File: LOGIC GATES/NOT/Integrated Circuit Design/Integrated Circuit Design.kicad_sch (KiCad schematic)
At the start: 13 parts, among them J1 Conn_01x03_Socket, J2 Conn_01x03_Socket, J3 Conn_01x03_Socket, Q1 QM6006D, Q2 QM6006D, Q3 QM6006D, U1 4011

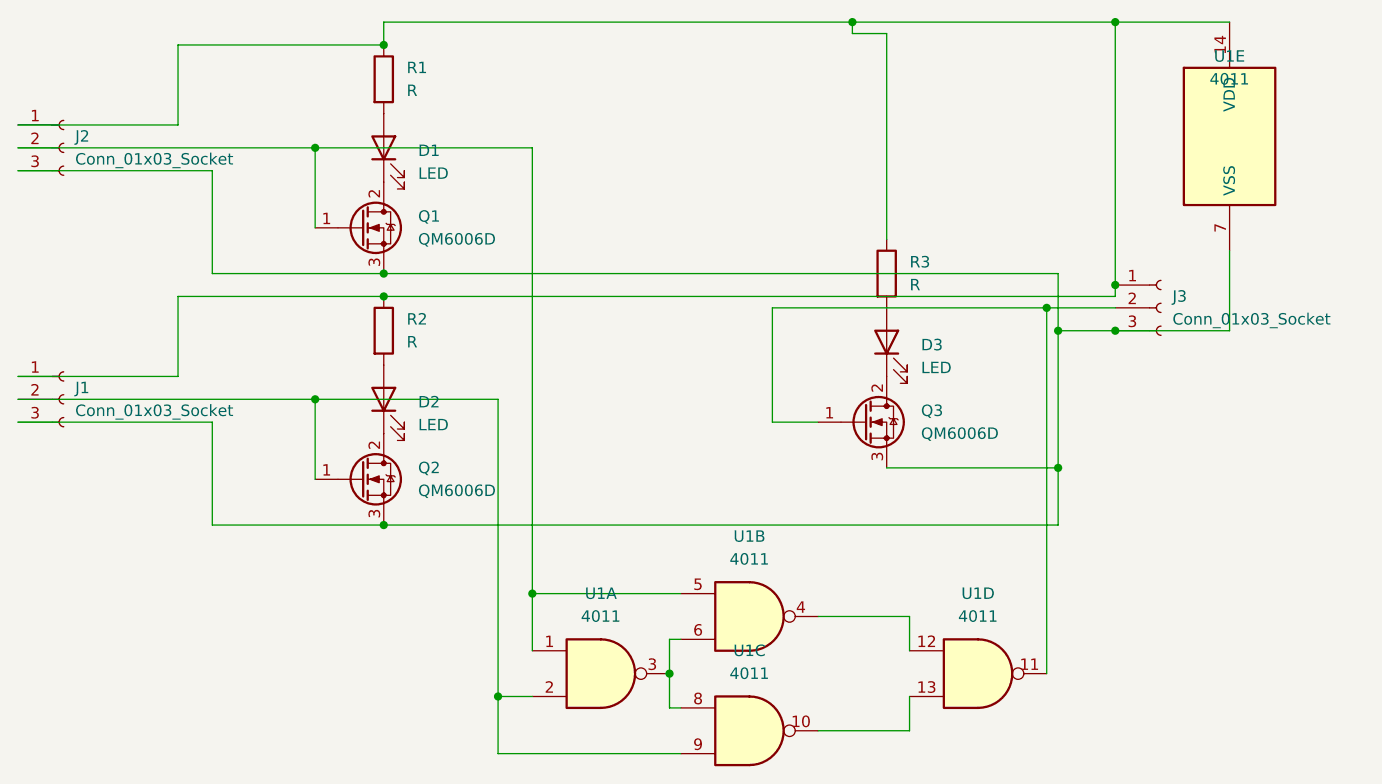
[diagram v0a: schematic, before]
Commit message: Auto-update: 21.12.2025 13:35:58,67
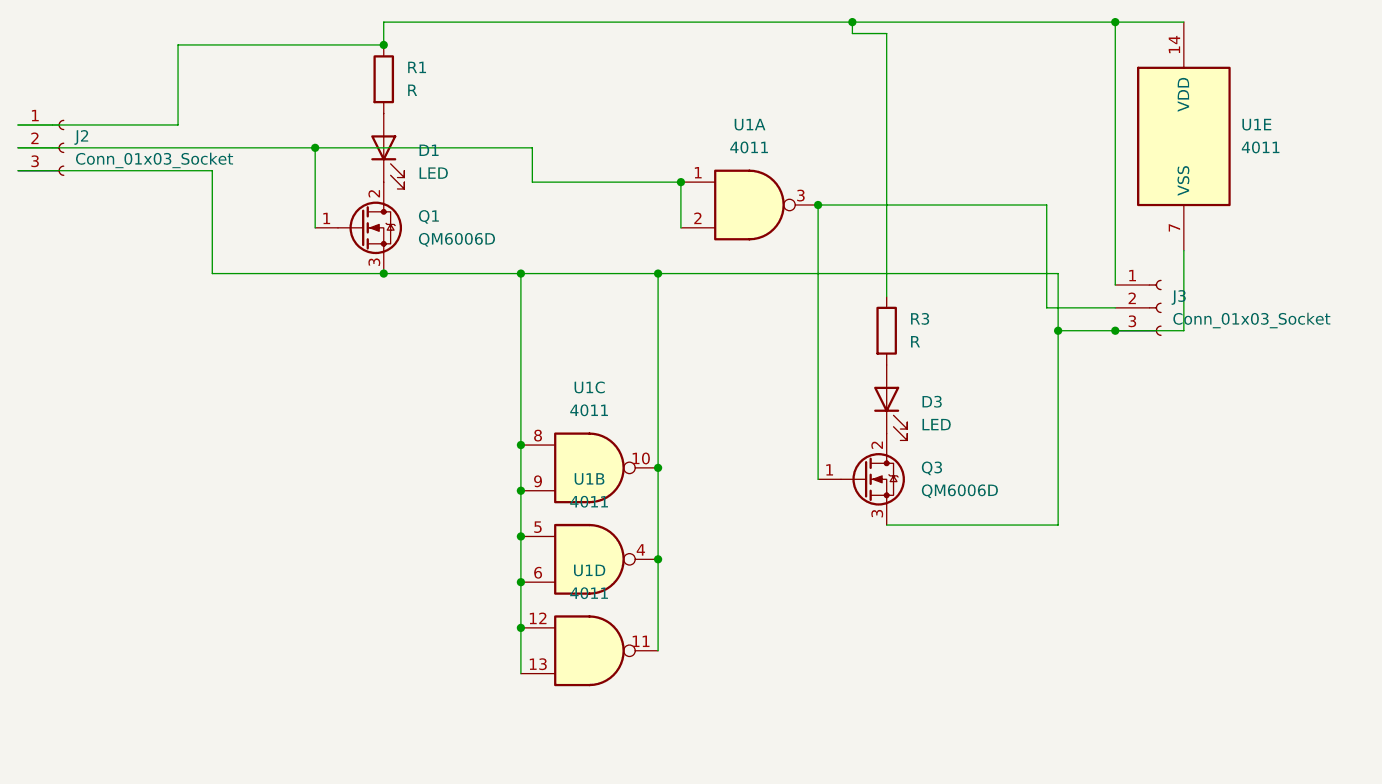
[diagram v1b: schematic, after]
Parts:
- removed D2: LED, LED_SMD:LED_1206_3216Metric, symbol Device:LED
- removed J1: Conn_01x03_Socket, Connector_PinSocket_2.54mm:PinSocket_1x03_P2.54mm_Horizontal, symbol Connector:Conn_01x03_Socket
- removed Q2: QM6006D, Package_TO_SOT_SMD:TO-252-2, symbol Transistor_FET:QM6006D
- removed R2: R, Resistor_SMD:R_1206_3216Metric, symbol Device:R
- U1: footprint (none) -> Package_DIP:DIP-14_W7.62mm
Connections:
- net at J2.2 (Pin_2), Q1.1 (G), U1.1: now also U1.2; no longer U1.5
- net at U1.9: now also J2.3 (Pin_3), J3.3 (Pin_3), Q1.3 (S), Q3.3 (S), U1.10, U1.11, U1.12, U1.13, U1.4, U1.5, U1.6, U1.7 (VSS), U1.8; no longer U1.2
- net at J3.2 (Pin_2), Q3.1 (G): now also U1.3; no longer U1.11
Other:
- moved on the sheet: D3, Q3, R3, U1A
